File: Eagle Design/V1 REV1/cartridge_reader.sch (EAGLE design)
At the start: 21 parts, among them IC1 AT90USB1287-AU

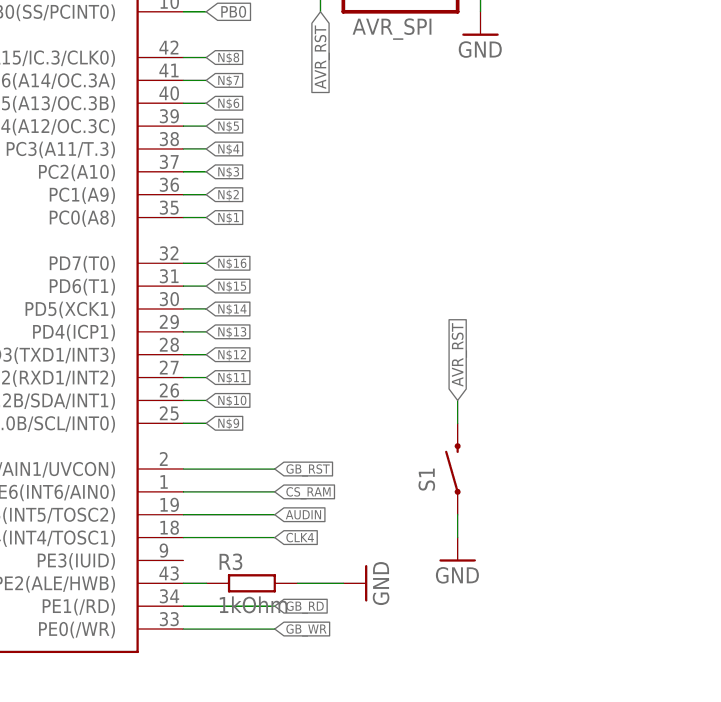
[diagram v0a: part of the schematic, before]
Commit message: lufa and cartridge dumper
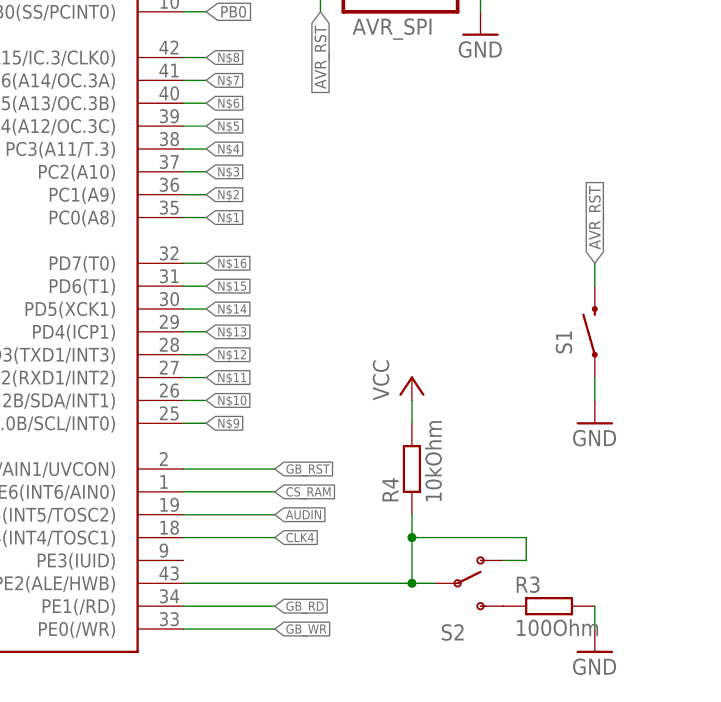
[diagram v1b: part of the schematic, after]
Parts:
- added R4: 10kOhm, rcl:R-EU_R0603
- added S2: (no value), SparkFun-Electromechanical:SWITCH-SPDT-SMD-A
- R3: value 1kOhm -> 100Ohm
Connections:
- new net N$43: R3.1, S2.S
- net N$26: now also R4.1, S2.O, S2.P; no longer R3.1
- net VCC: now also R4.2
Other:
- moved on the sheet: R3, S1
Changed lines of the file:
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@@
 <part name="P+3" library="supply1" deviceset="VCC" device=""/>
 <part name="GND2" library="supply1" deviceset="GND" device=""/>
-<part name="R3" library="rcl" deviceset="R-EU_" device="R0603" value="1kOhm"/>
+<part name="R3" library="rcl" deviceset="R-EU_" device="R0603" value="100Ohm"/>
 <part name="GND3" library="supply1" deviceset="GND" device=""/>
 <part name="C2" library="rcl" deviceset="C-EU" device="C0805K" value="0.1uF"/>
@@
 <part name="RN1" library="resistor-dil" deviceset="4R-N" device="0603-ARC"/>
 <part name="GND16" library="supply1" deviceset="GND" device=""/>
+<part name="S2" library="SparkFun-Electromechanical" deviceset="SWITCH-SPDT" device="-SMD-A"/>
+<part name="R4" library="rcl" deviceset="R-EU_" device="R0603" value="10kOhm"/>
+<part name="P+12" library="supply1" deviceset="VCC" device=""/>
 </parts>
 <sheets>
@@
 <instance part="P+3" gate="VCC" x="281.94" y="73.66" rot="R270"/>
 <instance part="GND2" gate="1" x="276.86" y="63.5"/>
-<instance part="R3" gate="G$1" x="251.46" y="2.54"/>
-<instance part="GND3" gate="1" x="264.16" y="2.54" rot="R90"/>
+<instance part="R3" gate="G$1" x="284.48" y="0"/>
+<instance part="GND3" gate="1" x="289.56" y="-5.08"/>
 <instance part="C2" gate="G$1" x="137.16" y="27.94"/>
 <instance part="GND10" gate="1" x="137.16" y="17.78"/>
@@
 <instance part="DM" gate="G$1" x="154.94" y="48.26"/>
 <instance part="DP" gate="G$1" x="149.86" y="50.8"/>
-<instance part="S1" gate="G$1" x="274.32" y="15.24" smashed="yes" rot="R90">
-<attribute name="NAME" x="271.78" y="12.7" size="1.778" layer="95" rot="R90"/>
+<instance part="S1" gate="G$1" x="289.56" y="30.48" smashed="yes" rot="R90">
+<attribute name="NAME" x="287.02" y="27.94" size="1.778" layer="95" rot="R90"/>
 </instance>
-<instance part="GND13" gate="1" x="274.32" y="5.08"/>
+<instance part="GND13" gate="1" x="289.56" y="20.32"/>
 <instance part="GND14" gate="1" x="127" y="81.28"/>
 <instance part="P+11" gate="VCC" x="127" y="88.9"/>
@@
 <instance part="RN1" gate="D" x="294.64" y="88.9" rot="R90"/>
 <instance part="GND16" gate="1" x="294.64" y="99.06" rot="R180"/>
+<instance part="S2" gate="1" x="274.32" y="2.54"/>
+<instance part="R4" gate="G$1" x="269.24" y="15.24" rot="R90"/>
+<instance part="P+12" gate="VCC" x="269.24" y="25.4"/>
 </instances>
 <busses>
@@
 <pinref part="R3" gate="G$1" pin="2"/>
 <pinref part="GND3" gate="1" pin="GND"/>
-<wire x1="261.62" y1="2.54" x2="256.54" y2="2.54" width="0.1524" layer="91"/>
+<wire x1="289.56" y1="-2.54" x2="289.56" y2="0" width="0.1524" layer="91"/>
 </segment>
 <segment>
@@
 <pinref part="S1" gate="G$1" pin="1"/>
 <pinref part="GND13" gate="1" pin="GND"/>
-<wire x1="274.32" y1="10.16" x2="274.32" y2="7.62" width="0.1524" layer="91"/>
+<wire x1="289.56" y1="25.4" x2="289.56" y2="22.86" width="0.1524" layer="91"/>
 </segment>
 <segment>
@@
 <pinref part="JP5" gate="G$1" pin="1"/>
 </segment>
+<segment>
+<pinref part="R4" gate="G$1" pin="2"/>
+<wire x1="269.24" y1="20.32" x2="269.24" y2="22.86" width="0.1524" layer="91"/>
+<pinref part="P+12" gate="VCC" pin="VCC"/>
+</segment>
 </net>
 <net name="N$1" class="0">
@@
 <segment>
 <pinref part="S1" gate="G$1" pin="2"/>
-<wire x1="274.32" y1="20.32" x2="274.32" y2="22.86" width="0.1524" layer="91"/>
-<label x="274.32" y="22.86" size="1.27" layer="95" rot="R90" xref="yes"/>
+<wire x1="289.56" y1="35.56" x2="289.56" y2="38.1" width="0.1524" layer="91"/>
+<label x="289.56" y="38.1" size="1.27" layer="95" rot="R90" xref="yes"/>
 </segment>
 </net>
@@
 <segment>
 <pinref part="IC1" gate="G$1" pin="PE2(ALE/HWB)"/>
-<pinref part="R3" gate="G$1" pin="1"/>
-<wire x1="246.38" y1="2.54" x2="243.84" y2="2.54" width="0.1524" layer="91"/>
+<pinref part="S2" gate="1" pin="P"/>
+<wire x1="271.78" y1="2.54" x2="269.24" y2="2.54" width="0.1524" layer="91"/>
+<wire x1="269.24" y1="2.54" x2="243.84" y2="2.54" width="0.1524" layer="91"/>
+<wire x1="269.24" y1="2.54" x2="269.24" y2="7.62" width="0.1524" layer="91"/>
+<pinref part="R4" gate="G$1" pin="1"/>
+<pinref part="S2" gate="1" pin="O"/>
+<wire x1="269.24" y1="7.62" x2="269.24" y2="10.16" width="0.1524" layer="91"/>
+<wire x1="279.4" y1="5.08" x2="281.94" y2="5.08" width="0.1524" layer="91"/>
+<wire x1="281.94" y1="5.08" x2="281.94" y2="7.62" width="0.1524" layer="91"/>
+<wire x1="281.94" y1="7.62" x2="269.24" y2="7.62" width="0.1524" layer="91"/>
+<junction x="269.24" y="2.54"/>
+<junction x="269.24" y="7.62"/>
 </segment>
 </net>
@@
 </segment>
 </net>
+<net name="N$43" class="0">
+<segment>
+<pinref part="S2" gate="1" pin="S"/>
+<pinref part="R3" gate="G$1" pin="1"/>
+</segment>
+</net>
